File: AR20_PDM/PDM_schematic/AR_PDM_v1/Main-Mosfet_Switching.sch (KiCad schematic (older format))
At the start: 57 parts, among them SW1 SW_DIP_x07, U15 NMOS, U16 NMOS, U17 NMOS, U18 NMOS, U19 NMOS, U20 NMOS, U21 NMOS, U22 NMOS, U23 NMOS, U24 NMOS, U25 NMOS, U26 NMOS, U27 NMOS, U28 NMOS

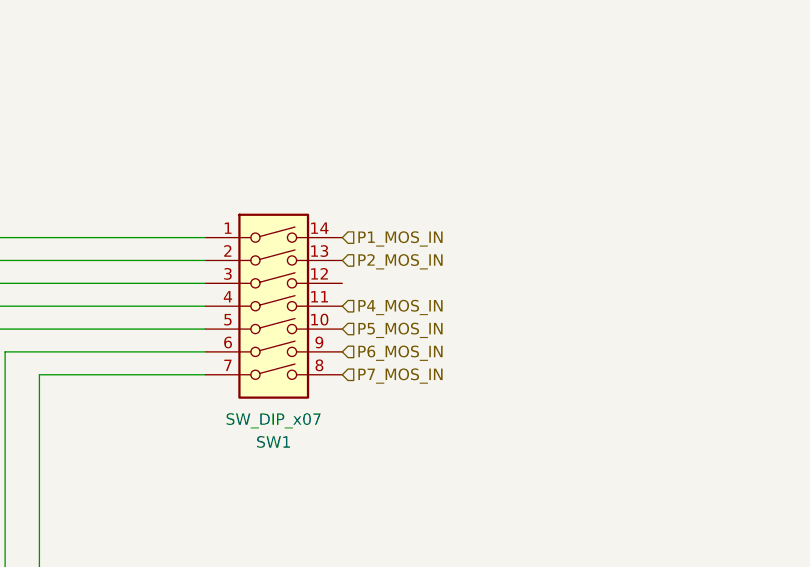
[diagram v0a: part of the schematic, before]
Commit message: Pdm version B Draft finished
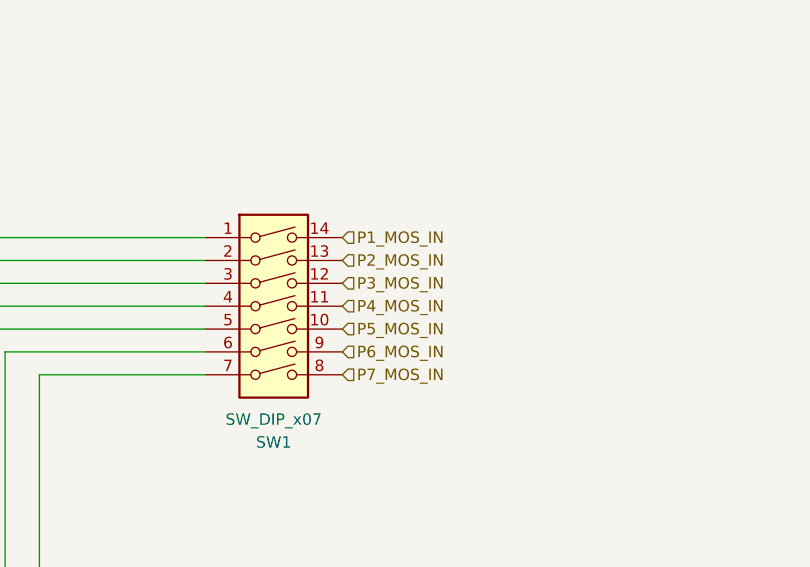
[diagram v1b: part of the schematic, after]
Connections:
- net P3_MOS_IN: now also SW1.12
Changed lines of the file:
@@
 Text HLabel 5700 1200 2    50   Input ~ 0
 P2_MOS_IN
-Text HLabel 5700 1400 2    50   Input ~ 0
-P4_MOS_IN
 Text HLabel 5700 1500 2    50   Input ~ 0
 P5_MOS_IN
@@
 Wire Wire Line
 	5100 1100 3625 1100
+Text HLabel 5700 1400 2    50   Input ~ 0
+P4_MOS_IN
+Text HLabel 5700 1300 2    50   Input ~ 0
+P3_MOS_IN
 $EndSCHEMATC
